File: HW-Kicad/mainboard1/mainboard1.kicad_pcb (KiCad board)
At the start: 2 copper layers, 33.6 x 63.4 mm, 1 part, among them M1 LightAPRS

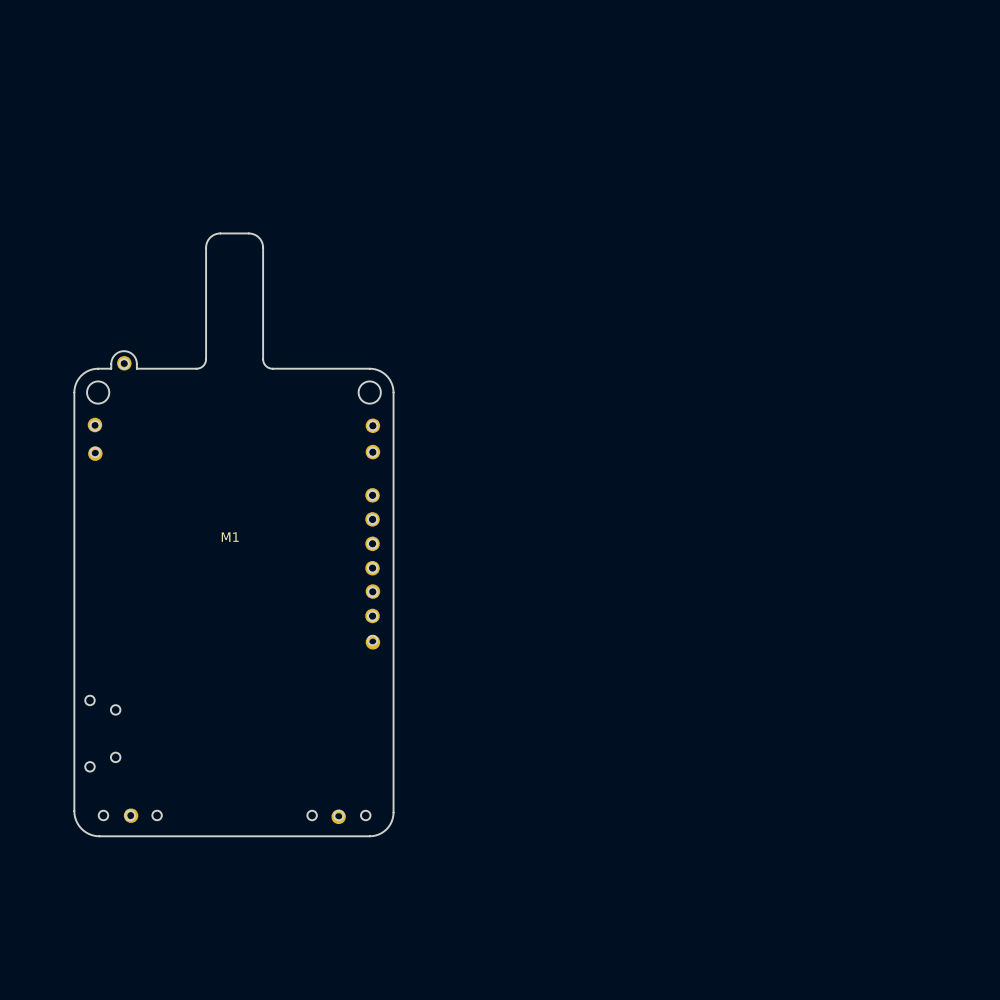
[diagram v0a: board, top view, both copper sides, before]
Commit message: comienzo mainboard
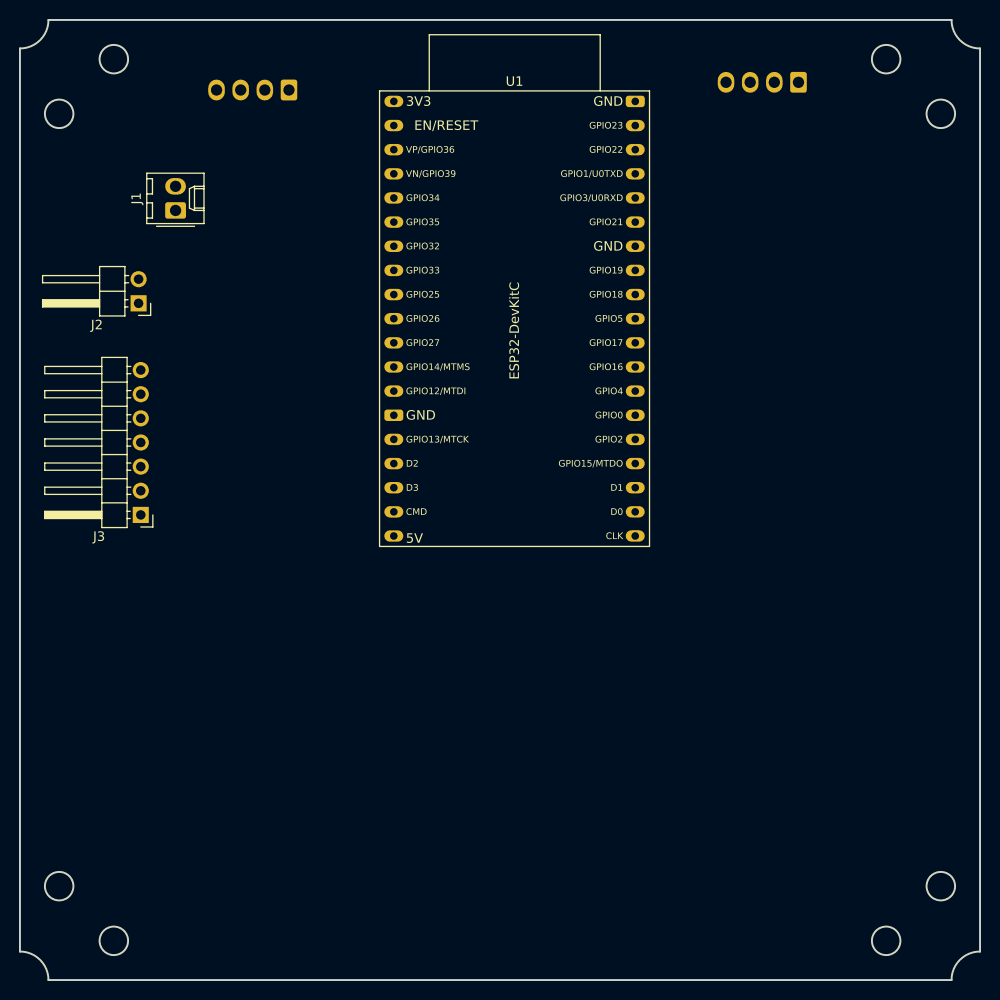
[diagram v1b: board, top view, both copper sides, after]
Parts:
- removed M1: LightAPRS, LightAPRS:LightAPRS
- added J1: Conn_01x02_Male, Connector_Molex:Molex_KK-254_AE-6410-02A_1x02_P2.54mm_Vertical, F.Cu at (132.6, 59.7)
- added J2: Conn_01x02_Male, Connector_PinHeader_2.54mm:PinHeader_1x02_P2.54mm_Horizontal, F.Cu at (128.7, 69.5)
- added J3: Conn_01x07_Male, Connector_PinHeader_2.54mm:PinHeader_1x07_P2.54mm_Horizontal, F.Cu at (128.9, 91.8)
- added J4: Conn_01x04_Male, Connector_Molex:Molex_KK-254_AE-6410-04A_1x04_P2.54mm_Vertical, B.Cu at (144.5, 47.1)
- added J5: Conn_01x04_Male, Connector_Molex:Molex_KK-254_AE-6410-04A_1x04_P2.54mm_Vertical, B.Cu at (198.1, 46.3)
- added U1: ESP32-DevKitC, espressif:ESP32-DevKitC, F.Cu at (155.6, 48.3)
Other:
- board size 33.6 x 63.4 mm -> 101 x 101 mm
